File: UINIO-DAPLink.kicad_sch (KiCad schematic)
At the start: 45 parts, among them J1 扩展板串口 & 电源输出, J2 扩展板 JTAG 输出, J3 JTAG_nTRST 跳线选择, J4 3.3V 跳线选择, J5 扩展板 SWD 输入, J6 DAPLink 固件下载接口, J7 SWD 下载输出, U1 ME6211C33M5G, U2 STM32F103C8T6, Y1 8MHz

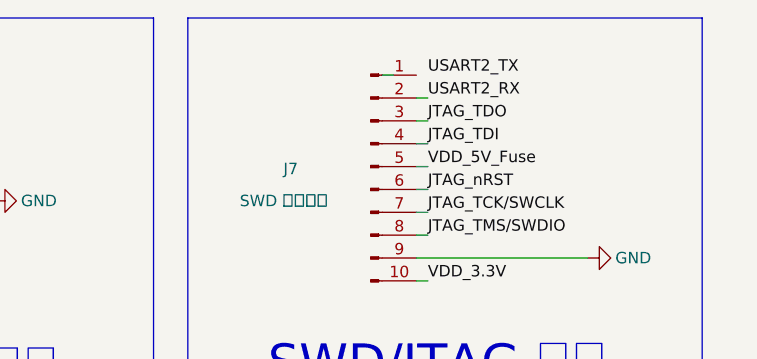
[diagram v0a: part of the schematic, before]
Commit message: update
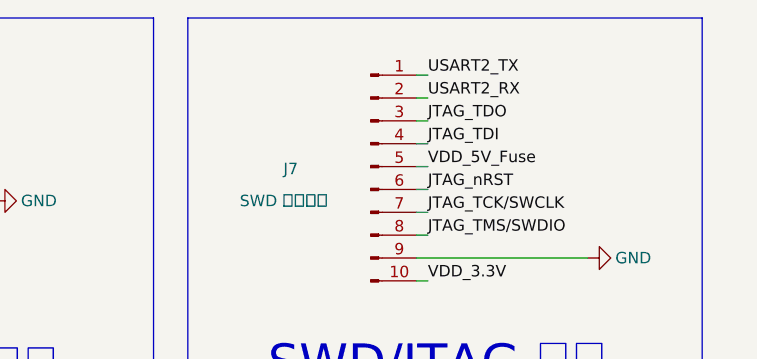
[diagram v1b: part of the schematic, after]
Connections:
- net USART2_TX: now also J7.1 (Pin_1)
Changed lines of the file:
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@@
 	(wire
 		(pts
-			(xy 245.11 22.86) (xy 243.84 22.86)
+			(xy 248.92 22.86) (xy 247.65 22.86)
 		)
 		(stroke
